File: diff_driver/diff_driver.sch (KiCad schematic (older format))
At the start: 14 parts, among them J1 CONN_01X07, J2 RJ45_LED, U1 am26ls31, U2 HT7533-1

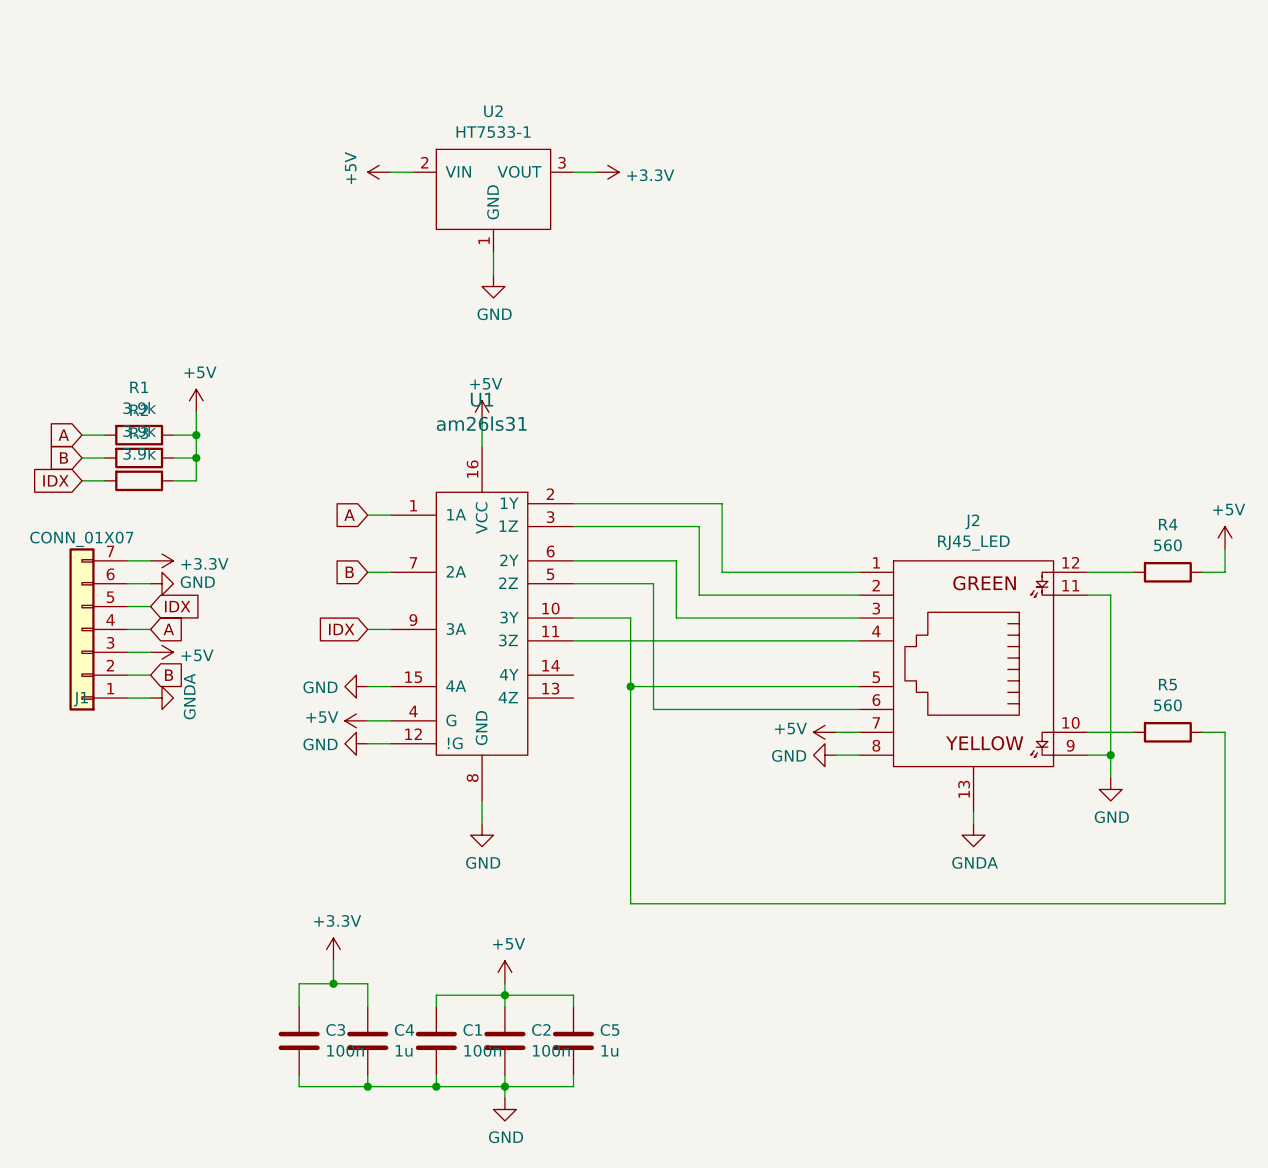
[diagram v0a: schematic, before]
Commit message: hw
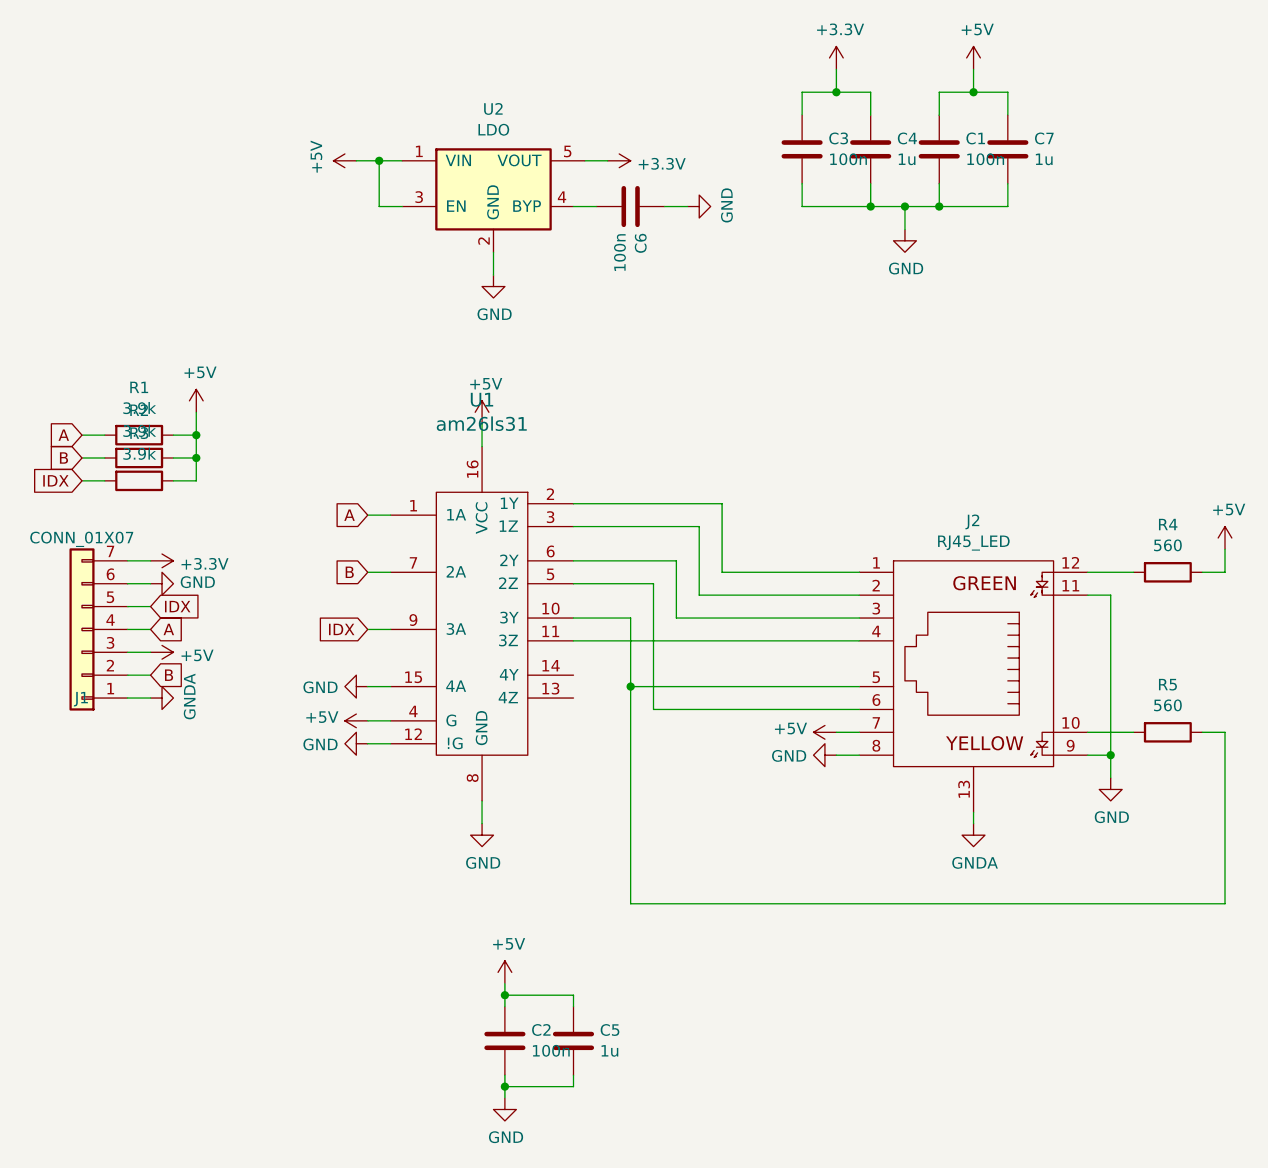
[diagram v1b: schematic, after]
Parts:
- removed U2: HT7533-1, stmbl:SOT-89-3, symbol stmbl:HT75XX-1
- added C6: 100n, stmbl:C_0603, symbol stmbl:C
- added C7: 1u, stmbl:C_0603, symbol stmbl:C
- added U2: LDO, stmbl:SOT-23-5, symbol stmbl:LDO
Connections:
- net +3V3: now also U2.5 (VOUT)
- net +5V: now also C7.1, U2.1 (VIN), U2.3 (EN)
- net GND: now also C6.1, C7.2, U2.2 (GND)
- new net: C6.2, U2.4 (BYP)
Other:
- moved on the sheet: C1, C3, C4
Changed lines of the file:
@@
 EESchema Schematic File Version 4
+LIBS:diff_driver-cache
 EELAYER 30 0
 EELAYER END
@@
 L stmbl:C C1
 U 1 1 5C799546
-P 4850 5800
-F 0 "C1" H 4965 5846 50  0000 L CNN
-F 1 "100n" H 4965 5755 50  0000 L CNN
-F 2 "stmbl:C_0603" H 4888 5650 50  0001 C CNN
-F 3 "~" H 4850 5800 50  0001 C CNN
-	1    4850 5800
+P 7050 1900
+F 0 "C1" H 7165 1946 50  0000 L CNN
+F 1 "100n" H 7165 1855 50  0000 L CNN
+F 2 "stmbl:C_0603" H 7088 1750 50  0001 C CNN
+F 3 "~" H 7050 1900 50  0001 C CNN
+	1    7050 1900
 	1    0    0    -1
 $EndComp
@@
 $EndComp
 Wire Wire Line
-	4850 5650 4850 5600
-Wire Wire Line
-	4850 5600 5150 5600
+	7050 1750 7050 1650
+Wire Wire Line
+	7050 1650 7200 1650
 Wire Wire Line
 	5450 5600 5450 5650
@@
 	5150 5550 5150 5600
 Wire Wire Line
-	4850 5950 4850 6000
-Wire Wire Line
-	4850 6000 5150 6000
+	7050 2050 7050 2150
+Wire Wire Line
+	7050 2150 7350 2150
 Wire Wire Line
 	5450 6000 5450 5950
@@
 L stmbl:+5V #PWR0116
 U 1 1 5DD62643
-P 4650 2000
-F 0 "#PWR0116" H 4650 1850 50  0001 C CNN
-F 1 "+5V" H 4665 2173 50  0000 C CNN
-F 2 "" H 4650 2000 50  0001 C CNN
-F 3 "" H 4650 2000 50  0001 C CNN
-	1    4650 2000
+P 4500 1950
+F 0 "#PWR0116" H 4500 1800 50  0001 C CNN
+F 1 "+5V" H 4515 2123 50  0000 C CNN
+F 2 "" H 4500 1950 50  0001 C CNN
+F 3 "" H 4500 1950 50  0001 C CNN
+	1    4500 1950
 	0    -1   -1   0
 $EndComp
 Wire Wire Line
-	4650 2000 4750 2000
+	4500 1950 4600 1950
 Wire Wire Line
 	5100 2450 5100 2350
@@
 L stmbl:+3.3V #PWR0117
 U 1 1 5DD66098
-P 5550 2000
-F 0 "#PWR0117" H 5550 1850 50  0001 C CNN
-F 1 "+3.3V" V 5565 2128 50  0000 L CNN
-F 2 "" H 5550 2000 50  0001 C CNN
-F 3 "" H 5550 2000 50  0001 C CNN
-	1    5550 2000
-	0    1    1    0
-$EndComp
-Wire Wire Line
-	5450 2000 5550 2000
-$Comp
-L stmbl:HT75XX-1 U2
-U 1 1 5DD6ED30
-P 5100 2000
-F 0 "U2" H 5100 2265 50  0000 C CNN
-F 1 "HT7533-1" H 5100 2174 50  0000 C CNN
-F 2 "stmbl:SOT-89-3" H 5100 2000 50  0001 C CNN
-F 3 "" H 5100 2000 50  0001 C CNN
-	1    5100 2000
-	1    0    0    -1
-$EndComp
+P 5600 1950
+F 0 "#PWR0117" H 5600 1800 50  0001 C CNN
+F 1 "+3.3V" V 5615 2078 50  0000 L CNN
+F 2 "" H 5600 1950 50  0001 C CNN
+F 3 "" H 5600 1950 50  0001 C CNN
+	1    5600 1950
+	0    1    1    0
+$EndComp
+Wire Wire Line
+	5500 1950 5600 1950
 $Comp
 L stmbl:+3.3V #PWR0118
@@
 L stmbl:C C4
 U 1 1 5DD7DCEF
-P 4550 5800
-F 0 "C4" H 4665 5846 50  0000 L CNN
-F 1 "1u" H 4665 5755 50  0000 L CNN
-F 2 "stmbl:C_0603" H 4588 5650 50  0001 C CNN
-F 3 "~" H 4550 5800 50  0001 C CNN
-	1    4550 5800
-	1    0    0    -1
-$EndComp
-Wire Wire Line
-	4550 5950 4550 6000
-Wire Wire Line
-	4550 6000 4850 6000
-Connection ~ 4850 6000
+P 6750 1900
+F 0 "C4" H 6865 1946 50  0000 L CNN
+F 1 "1u" H 6865 1855 50  0000 L CNN
+F 2 "stmbl:C_0603" H 6788 1750 50  0001 C CNN
+F 3 "~" H 6750 1900 50  0001 C CNN
+	1    6750 1900
+	1    0    0    -1
+$EndComp
+Wire Wire Line
+	6750 2050 6750 2150
+Wire Wire Line
+	6750 2150 6900 2150
+Connection ~ 7050 2150
 $Comp
 L stmbl:+3.3V #PWR0119
 U 1 1 5DD815EC
-P 4400 5450
-F 0 "#PWR0119" H 4400 5300 50  0001 C CNN
-F 1 "+3.3V" H 4415 5623 50  0000 C CNN
-F 2 "" H 4400 5450 50  0001 C CNN
-F 3 "" H 4400 5450 50  0001 C CNN
-	1    4400 5450
-	1    0    0    -1
-$EndComp
-Wire Wire Line
-	4550 5550 4550 5650
+P 6600 1550
+F 0 "#PWR0119" H 6600 1400 50  0001 C CNN
+F 1 "+3.3V" H 6615 1723 50  0000 C CNN
+F 2 "" H 6600 1550 50  0001 C CNN
+F 3 "" H 6600 1550 50  0001 C CNN
+	1    6600 1550
+	1    0    0    -1
+$EndComp
+Wire Wire Line
+	6750 1650 6750 1750
 $Comp
 L stmbl:C C3
 U 1 1 5DD85645
-P 4250 5800
-F 0 "C3" H 4365 5846 50  0000 L CNN
-F 1 "100n" H 4365 5755 50  0000 L CNN
-F 2 "stmbl:C_0603" H 4288 5650 50  0001 C CNN
-F 3 "~" H 4250 5800 50  0001 C CNN
-	1    4250 5800
-	1    0    0    -1
-$EndComp
-Wire Wire Line
-	4550 6000 4250 6000
-Wire Wire Line
-	4250 6000 4250 5950
-Connection ~ 4550 6000
-Wire Wire Line
-	4250 5650 4250 5550
-Wire Wire Line
-	4250 5550 4400 5550
-Wire Wire Line
-	4400 5450 4400 5550
-Connection ~ 4400 5550
-Wire Wire Line
-	4400 5550 4550 5550
+P 6450 1900
+F 0 "C3" H 6565 1946 50  0000 L CNN
+F 1 "100n" H 6565 1855 50  0000 L CNN
+F 2 "stmbl:C_0603" H 6488 1750 50  0001 C CNN
+F 3 "~" H 6450 1900 50  0001 C CNN
+	1    6450 1900
+	1    0    0    -1
+$EndComp
+Wire Wire Line
+	6750 2150 6450 2150
+Wire Wire Line
+	6450 2150 6450 2050
+Connection ~ 6750 2150
+Wire Wire Line
+	6450 1750 6450 1650
+Wire Wire Line
+	6450 1650 6600 1650
+Wire Wire Line
+	6600 1550 6600 1650
+Connection ~ 6600 1650
+Wire Wire Line
+	6600 1650 6750 1650
 Wire Wire Line
 	5700 5200 5700 4250
@@
 Wire Wire Line
 	3600 4300 3500 4300
+$Comp
+L stmbl:LDO U2
+U 1 1 5E922A67
+P 5100 2050
+F 0 "U2" H 5100 2375 50  0000 C CNN
+F 1 "LDO" H 5100 2284 50  0000 C CNN
+F 2 "stmbl:SOT-23-5" H 5750 1800 50  0001 C CIN
+F 3 "" H 5100 2050 50  0000 C CNN
+	1    5100 2050
+	1    0    0    -1
+$EndComp
+Wire Wire Line
+	4700 2150 4600 2150
+Wire Wire Line
+	4600 2150 4600 1950
+Connection ~ 4600 1950
+Wire Wire Line
+	4600 1950 4700 1950
+$Comp
+L stmbl:C C6
+U 1 1 5E933CE9
+P 5700 2150
+F 0 "C6" H 5815 2196 50  0000 L CNN
+F 1 "100n" H 5815 2105 50  0000 L CNN
+F 2 "stmbl:C_0603" H 5738 2000 50  0001 C CNN
+F 3 "~" H 5700 2150 50  0001 C CNN
+	1    5700 2150
+	0    1    1    0
+$EndComp
+Wire Wire Line
+	5450 2150 5550 2150
+$Comp
+L stmbl:GND #PWR0122
+U 1 1 5E936D2D
+P 5950 2150
+F 0 "#PWR0122" H 5950 1900 50  0001 C CNN
+F 1 "GND" H 5955 1977 50  0000 C CNN
+F 2 "" H 5950 2150 50  0001 C CNN
+F 3 "" H 5950 2150 50  0001 C CNN
+	1    5950 2150
+	0    -1   -1   0
+$EndComp
+Wire Wire Line
+	5850 2150 5950 2150
+$Comp
+L stmbl:C C7
+U 1 1 5E949F87
+P 7350 1900
+F 0 "C7" H 7465 1946 50  0000 L CNN
+F 1 "1u" H 7465 1855 50  0000 L CNN
+F 2 "stmbl:C_0603" H 7388 1750 50  0001 C CNN
+F 3 "~" H 7350 1900 50  0001 C CNN
+	1    7350 1900
+	1    0    0    -1
+$EndComp
+$Comp
+L stmbl:+5V #PWR0123
+U 1 1 5E94A508
+P 7200 1550
+F 0 "#PWR0123" H 7200 1400 50  0001 C CNN
+F 1 "+5V" H 7215 1723 50  0000 C CNN
+F 2 "" H 7200 1550 50  0001 C CNN
+F 3 "" H 7200 1550 50  0001 C CNN
+	1    7200 1550
+	1    0    0    -1
+$EndComp
+Wire Wire Line
+	7350 1650 7350 1750
+Wire Wire Line
+	7350 2050 7350 2150
+$Comp
+L stmbl:GND #PWR0124
+U 1 1 5E94F91D
+P 6900 2250
+F 0 "#PWR0124" H 6900 2000 50  0001 C CNN
+F 1 "GND" H 6905 2077 50  0000 C CNN
+F 2 "" H 6900 2250 50  0001 C CNN
+F 3 "" H 6900 2250 50  0001 C CNN
+	1    6900 2250
+	1    0    0    -1
+$EndComp
+Wire Wire Line
+	6900 2250 6900 2150
+Connection ~ 6900 2150
+Wire Wire Line
+	6900 2150 7050 2150
+Wire Wire Line
+	7200 1550 7200 1650
+Connection ~ 7200 1650
+Wire Wire Line
+	7200 1650 7350 1650
 $EndSCHEMATC
